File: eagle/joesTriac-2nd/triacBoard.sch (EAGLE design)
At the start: 12 parts, among them IC2 LM311N, X1 87832-06

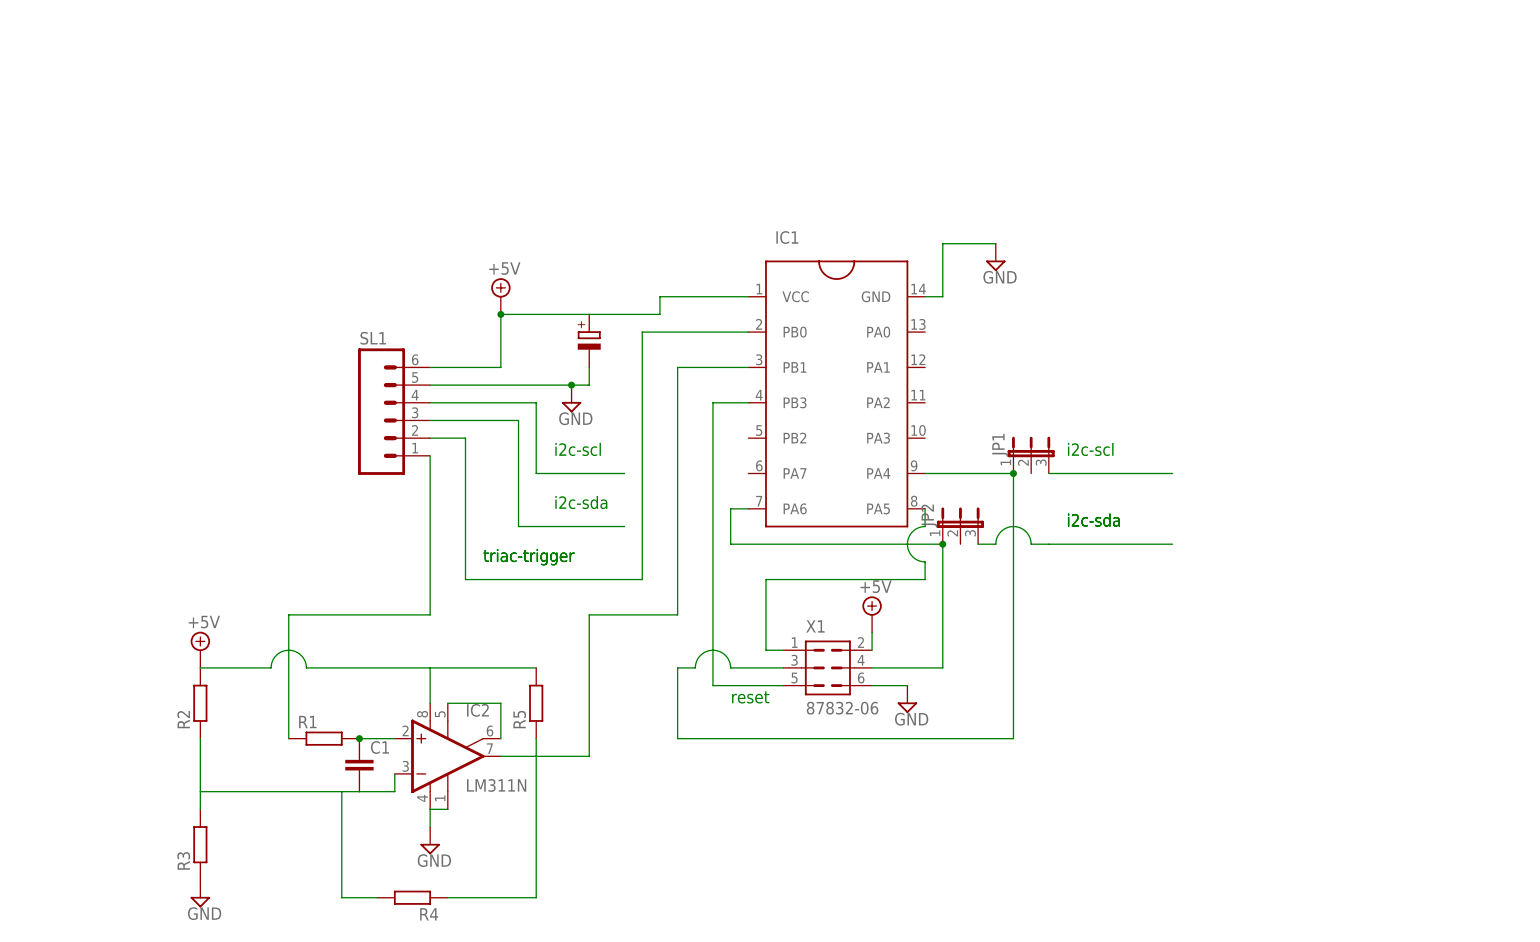
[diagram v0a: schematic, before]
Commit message: reg save
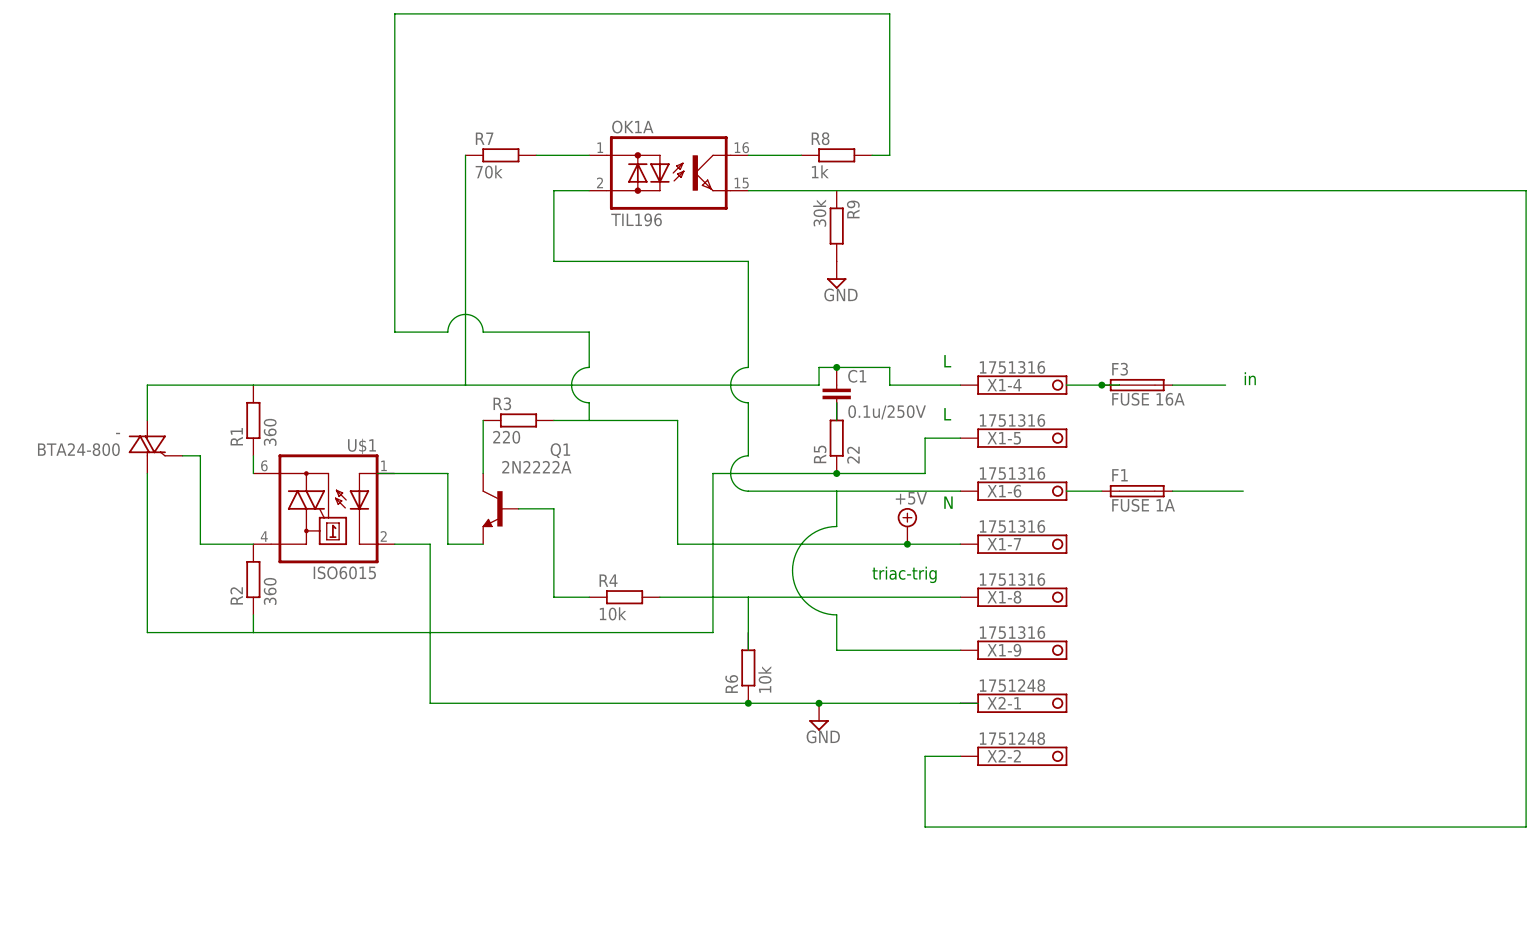
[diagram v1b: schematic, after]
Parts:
- removed IC1: (no value), atmel-new:ATTINY4414P3
- removed IC2: LM311N, linear:LM311N
- removed JP1, JP2: (no value), jumper:JP2E
- removed SL1: (no value), con-amp-quick:M06
- added -: BTA24-800, triac:BTA24-800
- added F1: FUSE 1A, fuse:FUSESH22,5
- added F3: FUSE 16A, fuse:FUSESH22,5
- added OK1: TIL196, optocoupler:TIL196
- added Q1: 2N2222A, transistor-npn:2N2222A
- added R6: 10k, resistor:R-EU_0207/15
- added R7: 70k, resistor:R-EU_0207/15
- added R8: 1k, resistor:R-EU_0207/15
- added R9: 30k, resistor:R-EU_0207/15
- added U$1: ISO6015, optocoupler:ISO6015
- added X2: 1751248, con-phoenix-350:1751248
- C1: value (none) -> 0.1u/250V; device capacitor-wima:C2,5-3 -> capacitor-wima:C5/5
- R1, R2: value (none) -> 360; device resistor:R-EU_0207/10 -> resistor:R-EU_0207/15
- R3: value (none) -> 220; device resistor:R-EU_0207/10 -> resistor:R-EU_0207/15
- R4: value (none) -> 10k; device resistor:R-EU_0207/10 -> resistor:R-EU_0207/15
- R5: value (none) -> 22; device resistor:R-EU_0207/10 -> resistor:R-EU_0309/12
- X1: value 87832-06 -> 1751316; device con-molex:87832-06 -> con-phoenix-350:1751316
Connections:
- removed net N$9: IC1.PB0, SL1.2
- new net N$15: OK1A.C, R8.1
- new net N$17: OK1A.E, X2-2.K
- new net N$19: F3.2
- new net N$21: OK1A.AC2, X1-6.K, X1-9.K
- net +5V: now also R3.2, R8.2, X1-7.K; no longer IC1.VCC, IC2.V+, R2.2, R5.2, SL1.6, X1.2
- net GND: now also R6.1, R9.2, U$1.C; no longer IC1.GND, IC2.GND, IC2.V-, R3.1, SL1.5, X1.6
- net N$1: now also OK1A.AC1, R7.2; no longer JP1.3
- net N$10: now also Q1.C, R3.1; no longer R1.1, SL1.1
- net N$11: now also Q1.E; no longer C1.1, IC2.+IN, R1.2
- net N$12: now also X1-8.K; no longer C1.2, IC2.-IN, R2.1, R3.2
- net N$13: now also Q1.B, R4.1; no longer IC2.ON, IC2.ON/STR
- net N$14: now also F3.1; no longer IC1.PB1, IC2.OUT, R4.1, R5.1
- net N$2: now also F1.2; no longer IC1.PA6, JP2.1, X1.4
- net N$3: now also F1.1; no longer IC1.PA5, X1.1
- net N$4: now also -.A2, C1.1, R1.2, R7.1, X1-4.K; no longer IC1.PB3, X1.5
- net N$5: now also -.A1, R2.1, R5.1, X1-5.K; no longer IC1.PA4, JP1.1, X1.3
- net N$6: now also R1.1, U$1.A2; no longer SL1.3
- net N$7: now also -.G, R2.2, U$1.A1; no longer JP2.3
- net N$8: now also C1.2, R5.2; no longer SL1.4
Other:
- note added: "L"
- note added: "N"
- note added: "in"
- note added: "triac-trig"
- note removed: "i2c-scl"
- note removed: "i2c-sda"
- note removed: "reset"
- note removed: "triac-trigger"
- moved on the sheet: C1, R1, R2, R3, R4, R5
